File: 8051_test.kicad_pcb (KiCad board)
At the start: 2 copper layers, 50 x 56 mm, 37 parts, among them J17 Prog, J2 Pwr, J24 Conn_01x20_Pin, J25 Conn_01x20_Pin, J4 Conn_02x09_Odd_Even, Q1 MMBT3906, Q2 MMBT3906, Q3 2N7002, Q4 Conn_02x02_Odd_Even, U1 8051, Y1 Crystal

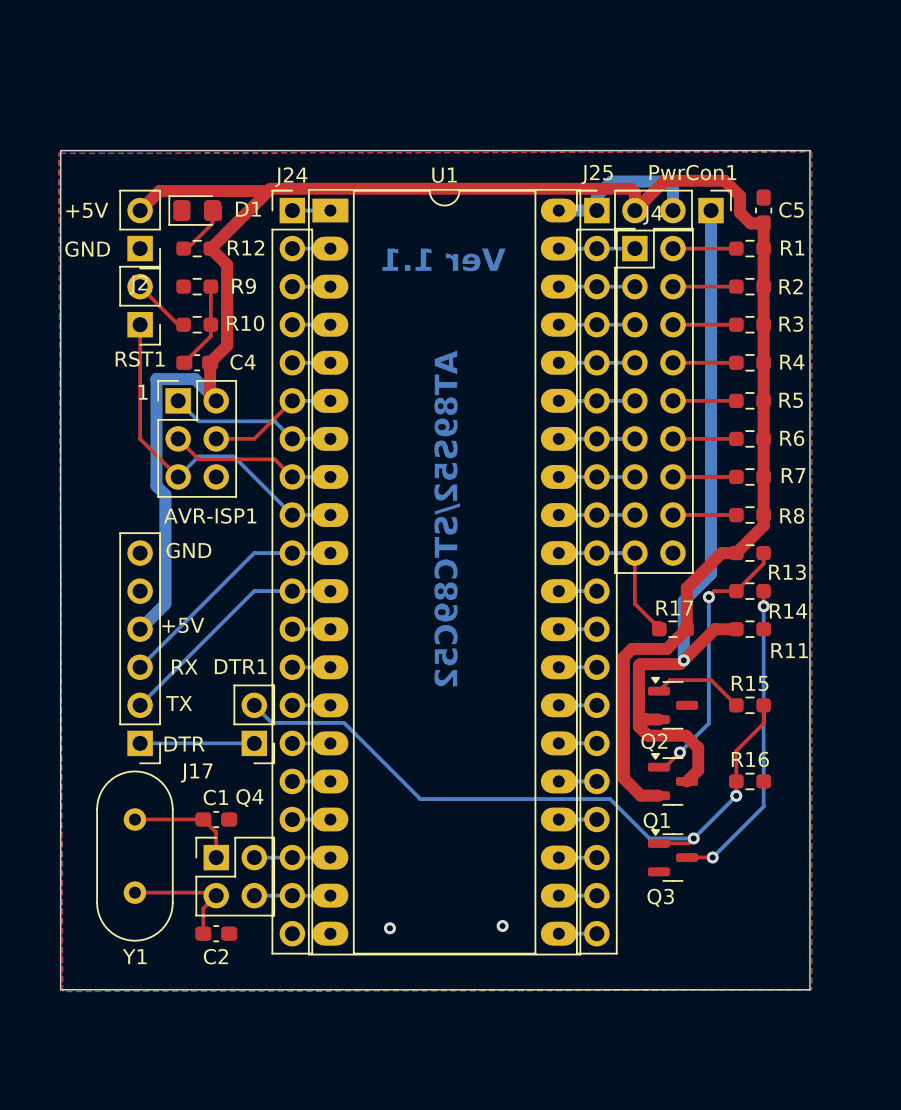
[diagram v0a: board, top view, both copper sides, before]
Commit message: Updated to next version using ZIF socket
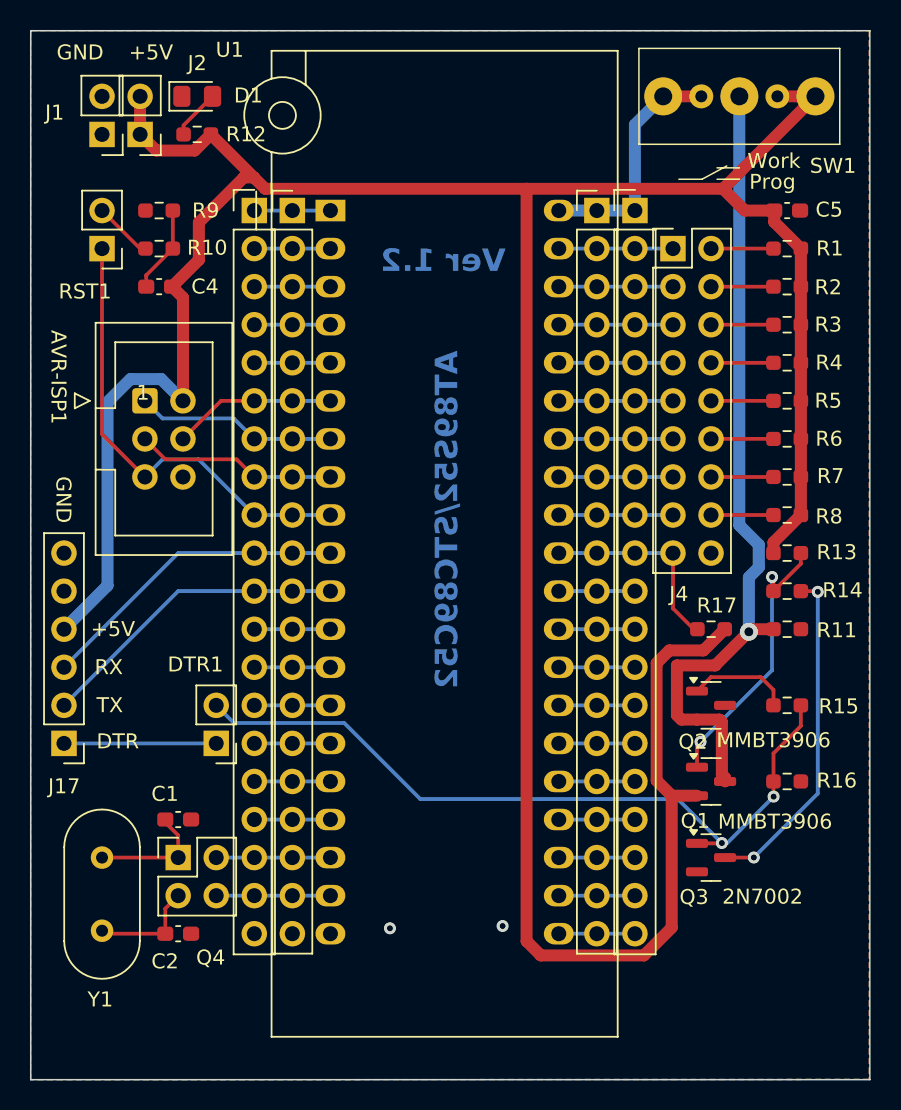
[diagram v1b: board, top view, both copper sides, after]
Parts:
- removed PwrCon1: Conn_01x03_Pin, Connector_PinHeader_2.54mm:PinHeader_1x03_P2.54mm_Vertical
- added J1: GND, Connector_PinHeader_2.54mm:PinHeader_1x02_P2.54mm_Vertical, F.Cu at (64.8, 54.9)
- added J3: PL2, Connector_PinHeader_2.54mm:PinHeader_1x20_P2.54mm_Vertical, F.Cu at (74.9, 60.0)
- added J5: PR2, Connector_PinHeader_2.54mm:PinHeader_1x20_P2.54mm_Vertical, F.Cu at (100.3, 60.0)
- added SW1: SW_SPDT, Button_Switch_THT:SPDT_Omron_D2F_5pins, F.Cu at (107.3, 52.4)
- AVR-ISP1: footprint Connector_PinHeader_2.54mm:PinHeader_2x03_P2.54mm_Vertical -> Connector_IDC:IDC-Header_2x03_P2.54mm_Vertical
- DTR1: value Conn_01x02_Pin -> Prog
- J17: value Prog -> UART
- J2: value Pwr -> +5V
- J24: value Conn_01x20_Pin -> PL1
- J25: value Conn_01x20_Pin -> PR1
- J4: value Conn_02x09_Odd_Even -> Rs
- Q4: value Conn_02x02_Odd_Even -> Conn Crystal
- RST1: value Conn_01x02_Pin -> Reset
- U1: footprint Package_DIP:DIP-40_W15.24mm_Socket_LongPads -> Socket:DIP_Socket-40_W11.9_W12.7_W15.24_W17.78_W18.5_3M_240-1280-00-0602J
- Y1: value Crystal -> 11.0592
- moved D1 7.62 mm to (71.1, 52.4)
- moved J2 7.62 mm to (67.3, 54.9)
- moved R12 7.62 mm to (71.1, 54.9)
- moved R10 5.68 mm to (68.6, 62.5)
- moved C4 5.68 mm to (68.6, 65.1)
- moved R9 5.68 mm to (68.6, 60.0)
- moved RST1 5.68 mm to (64.8, 62.5)
- moved J17 5.08 mm to (62.2, 95.6)
- moved Y1 3.36 mm to (64.8, 103.2)
- moved DTR1 2.54 mm to (72.4, 95.6)
- moved J4 2.54 mm to (102.9, 62.5)
- moved Q1 2.54 mm to (105.4, 98.1)
- moved Q2 2.54 mm to (105.4, 93.0)
- moved Q3 2.54 mm to (105.4, 103.2)
- moved R17 2.54 mm to (105.4, 87.9)
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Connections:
- net /RD renamed /~{RD}
- net /WR renamed /~{WR}
- J2 pad 1: GND -> +5V
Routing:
- net +5V: track 131.3 -> 210.3 mm
- net /RST: track 23.6 -> 30.8 mm
- net /VPP: track 10.7 -> 16.0 mm
- net /P3.0: track 15.9 -> 20.9 mm
- net /P3.1: track 15.9 -> 20.9 mm
- net Net-(DTR1-Pin_2): track 46.3 -> 50.8 mm
- net Net-(Q1-C): track 50.8 -> 54.5 mm
- net /X2: track 5.08 -> 7.90 mm
- net /X1: track 5.08 -> 7.62 mm
- net /AD7: track 5.08 -> 7.62 mm
- net /AD6: track 5.08 -> 7.62 mm
- net /AD5: track 5.08 -> 7.62 mm
- net /AD4: track 5.08 -> 7.62 mm
- net /AD3: track 5.08 -> 7.62 mm
- net /AD2: track 5.08 -> 7.62 mm
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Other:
- board size 50 x 56 mm -> 56 x 70 mm
- board text added: "Prog"
- board text added: "Ver 1.2"
- board text added: "Work"
- board text removed: "Ver 1.1"
